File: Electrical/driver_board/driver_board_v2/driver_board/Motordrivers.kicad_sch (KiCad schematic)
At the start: 30 parts, among them J4 Conn_01x04_Socket, J5 Conn_01x04_Socket, J6 Conn_01x04_Socket, J7 Conn_01x04_Socket, J8 Conn_01x04_Socket, J9 Conn_01x04_Socket

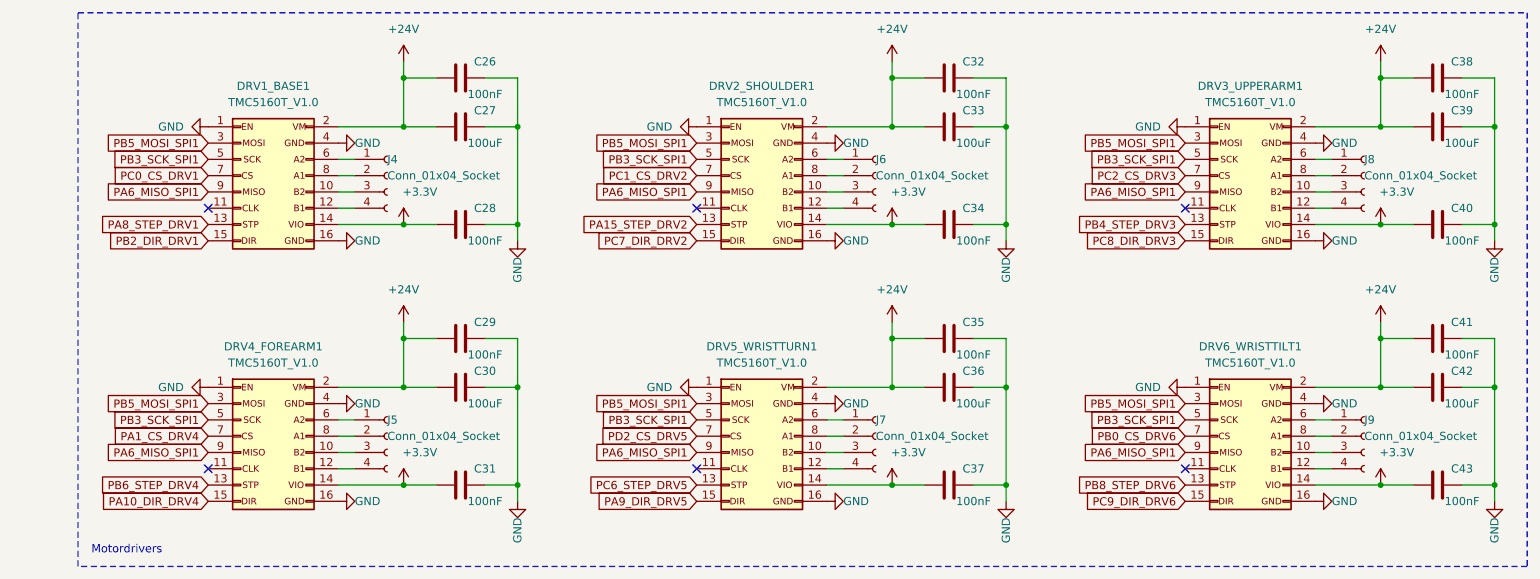
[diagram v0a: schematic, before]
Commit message: Pull up/downs
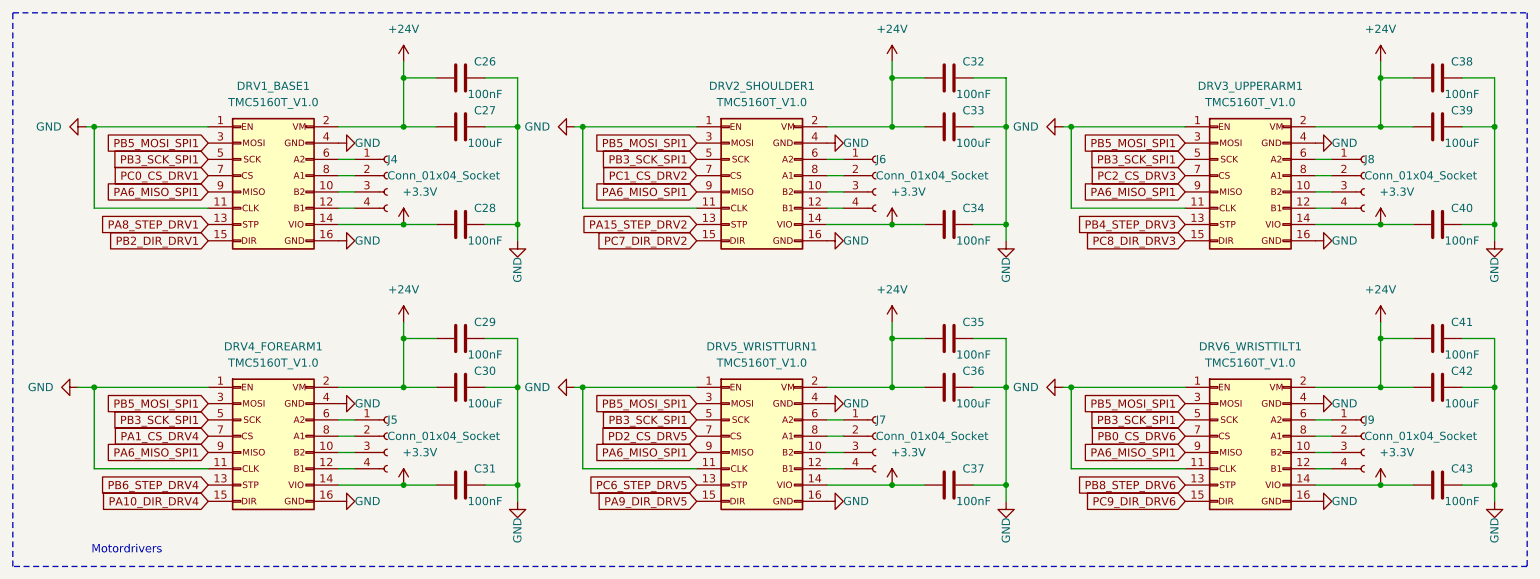
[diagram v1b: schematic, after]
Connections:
- net GND: now also DRV1_BASE1.11 (Pin_11), DRV2_SHOULDER1.11 (Pin_11), DRV3_UPPERARM1.11 (Pin_11), DRV4_FOREARM1.11 (Pin_11), DRV5_WRISTTURN1.11 (Pin_11), DRV6_WRISTTILT1.11 (Pin_11)
- no-connect marks 6 -> 0
